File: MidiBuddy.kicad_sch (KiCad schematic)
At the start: 8 parts, among them J1 MIDI OUT, J2 MIDI IN, U1 6N136

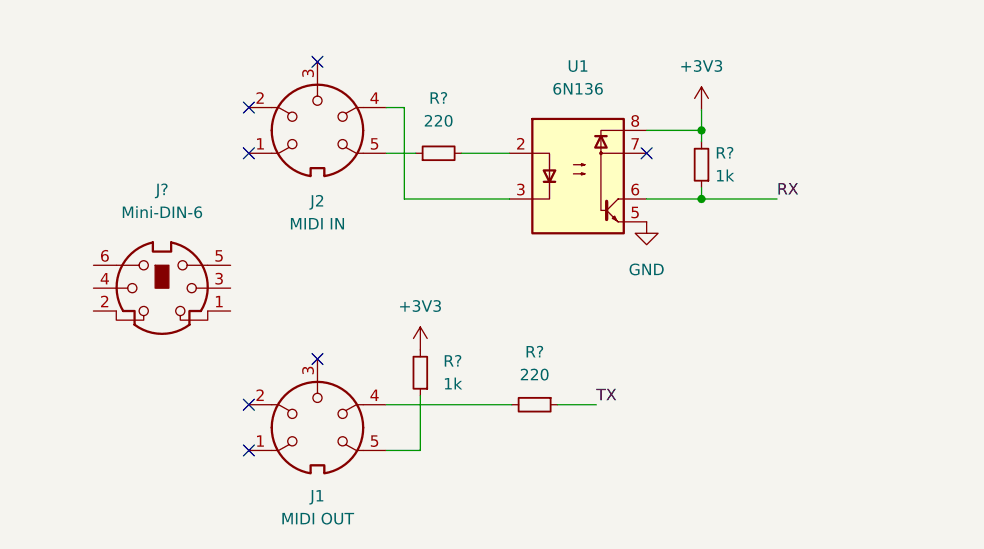
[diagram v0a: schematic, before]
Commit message: Initial pcb design
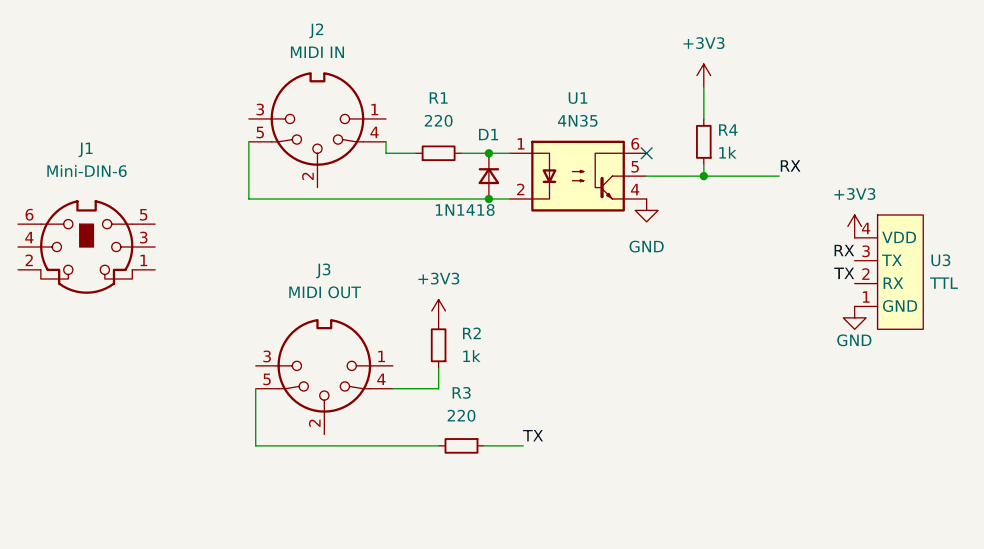
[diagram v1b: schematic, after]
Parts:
- removed J1: MIDI OUT, midi:midi, symbol Connector:DIN-5
- removed J2: MIDI IN, midi:midi, symbol Connector:DIN-5
- removed U1: 6N136, Package_DIP:DIP-8_W7.62mm_LongPads, symbol Isolator:6N136
- added D1: 1N1418, Diode_THT:D_A-405_P7.62mm_Horizontal, symbol Device:D_Small
- added J2: MIDI IN, midi:midi, symbol Connector:DIN-5_180degree
- added J3: MIDI OUT, midi:midi, symbol Connector:DIN-5_180degree
- added U1: 4N35, Package_DIP:DIP-6_W7.62mm, symbol Isolator:4N35
- added U3: TTL, Connector_PinHeader_2.54mm:PinHeader_1x04_P2.54mm_Vertical, symbol ftdi-connector:TTL
- gave numbers to parts that had none: 5
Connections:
- net +3V3: now also U3.4 (VDD)
- net GND: now also U1.4, U3.1 (GND)
- net RX: now also U1.5, U3.3 (TX)
- net TX: now also U3.2 (RX)
- net at R2.1: now also J3.4
- net at R1.1: now also J2.4
- net at R1.2: now also D1.1 (K), U1.1
- net at R3.2: now also J3.5
- new net: D1.2 (A), J2.5, U1.2
- no-connect marks 7 -> 1
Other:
- moved on the sheet: J1, R2, R3, R4
